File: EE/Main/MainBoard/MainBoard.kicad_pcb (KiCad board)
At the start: 2 copper layers, 141.8 x 89.6 mm, 18 parts, among them J1 Conn_02x13_Odd_Even, J2 Conn_02x13_Odd_Even, J3 Conn_02x13_Odd_Even, J4 Conn_02x13_Odd_Even, J5 Conn_02x13_Odd_Even

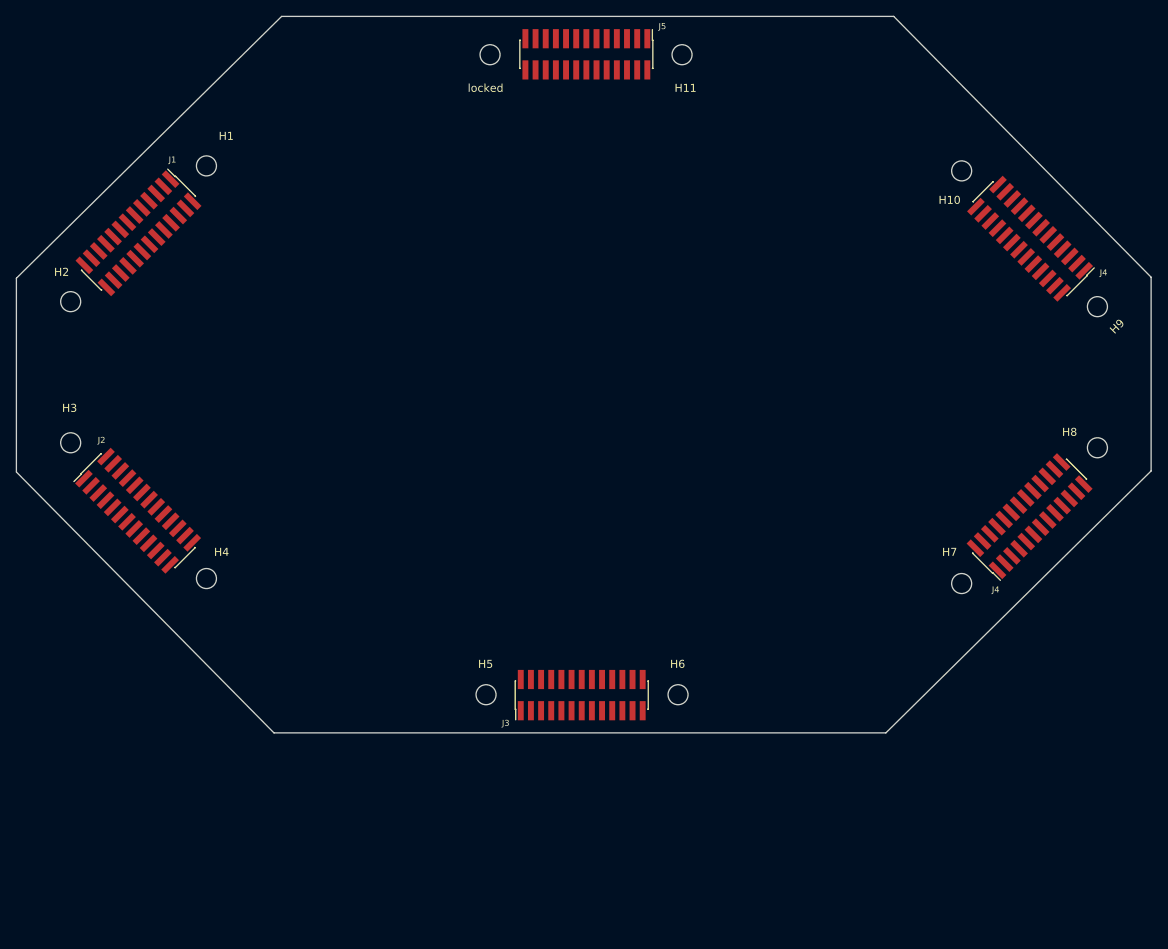
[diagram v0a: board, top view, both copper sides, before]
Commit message: Updated layout, and placement for main board
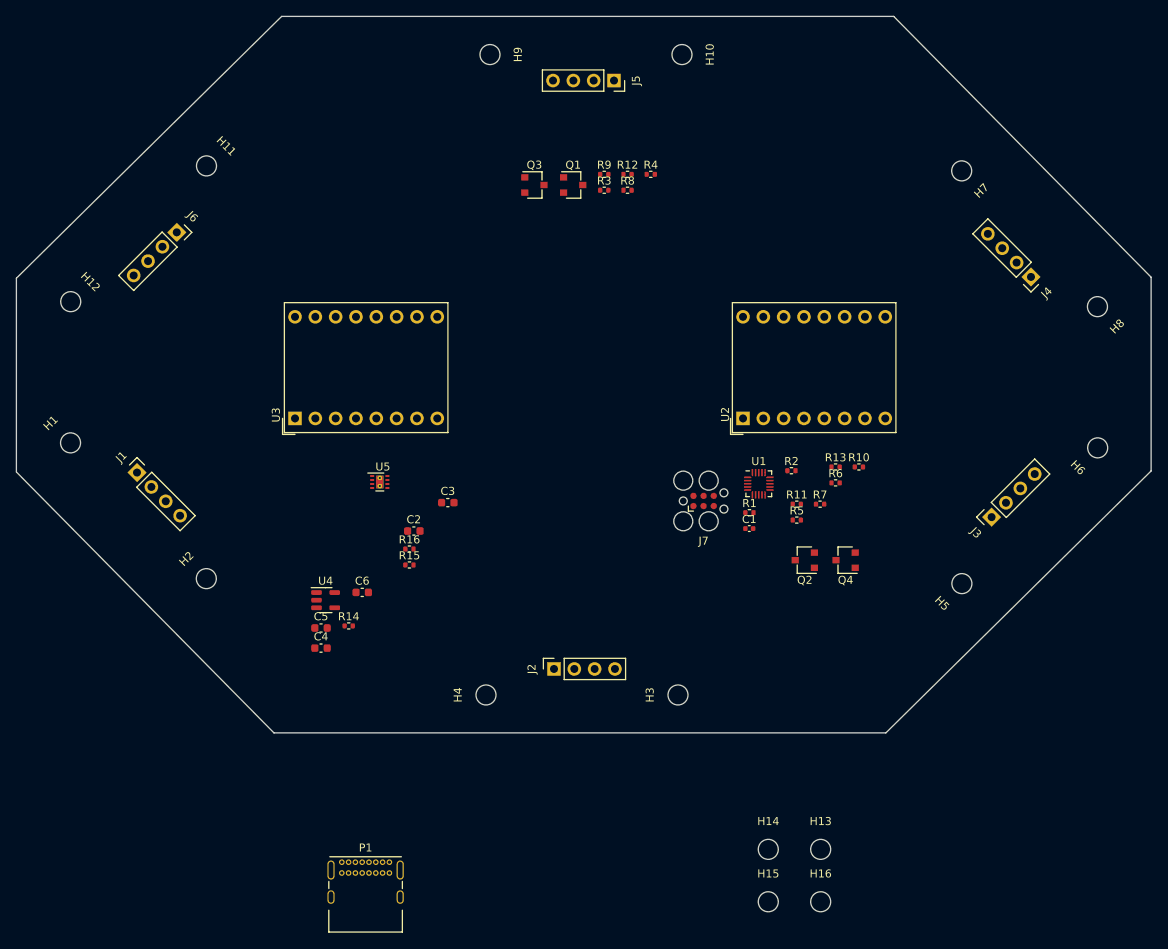
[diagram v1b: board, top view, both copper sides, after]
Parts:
- removed the J4 at (199.1, 77.8)
- removed the J4 at (199.0, 112.5)
- removed locked: MountingHole, MountingHole:MountingHole_2.5mm
- added C1: 0.1u, Capacitor_SMD:C_0402_1005Metric, F.Cu at (164.0, 114.0)
- added C2: 4.7u, Capacitor_SMD:C_0603_1608Metric, F.Cu at (122.0, 114.4)
- added C3: 4.7u, Capacitor_SMD:C_0603_1608Metric, F.Cu at (126.3, 110.8)
- added C4: 4.7u, Capacitor_SMD:C_0603_1608Metric, F.Cu at (110.4, 129.0)
- added C5: 4.7u, Capacitor_SMD:C_0603_1608Metric, F.Cu at (110.4, 126.5)
- added C6: 4.7u, Capacitor_SMD:C_0603_1608Metric, F.Cu at (115.6, 122.0)
- added H12: MountingHole, MountingHole:MountingHole_2.5mm, F.Cu at (79.1, 85.7)
- added H13: MountingHole, MountingHole:MountingHole_2.5mm, F.Cu at (172.9, 154.2)
- added H14: MountingHole, MountingHole:MountingHole_2.5mm, F.Cu at (166.3, 154.2)
- added H15: MountingHole, MountingHole:MountingHole_2.5mm, F.Cu at (166.3, 160.7)
- added H16: MountingHole, MountingHole:MountingHole_2.5mm, F.Cu at (172.9, 160.7)
- added J4: Conn_01x04_Male, Connector_PinSocket_2.54mm:PinSocket_1x04_P2.54mm_Vertical, F.Cu at (199.2, 82.6)
- added J6: Conn_01x04_Male, Connector_PinSocket_2.54mm:PinSocket_1x04_P2.54mm_Vertical, F.Cu at (92.4, 77.0)
- added J7: TAG_CONNECT, Connector:Tag-Connect_TC2030-IDC-FP_2x03_P1.27mm_Vertical, F.Cu at (158.2, 110.6)
- added P1: USB_C_Plug_USB2.0, Connector_USB:USB_C_Receptacle_GCT_USB4085, F.Cu at (113.0, 155.8)
- added Q1: 2N7002NXAKR, Package_TO_SOT_SMD:SC-59, F.Cu at (141.9, 71.1)
- added Q2: 2N7002NXAKR, Package_TO_SOT_SMD:SC-59, F.Cu at (170.9, 118.0)
- added Q3: 2N7002NXAKR, Package_TO_SOT_SMD:SC-59, F.Cu at (137.1, 71.1)
- added Q4: 2N7002NXAKR, Package_TO_SOT_SMD:SC-59, F.Cu at (176.0, 118.0)
- added R1: 4.7k, Resistor_SMD:R_0402_1005Metric, F.Cu at (164.0, 112.1)
- added R10: 560, Resistor_SMD:R_0402_1005Metric, F.Cu at (177.7, 106.3)
- added R11: 560, Resistor_SMD:R_0402_1005Metric, F.Cu at (169.9, 111.0)
- added R12: 560, Resistor_SMD:R_0402_1005Metric, F.Cu at (148.7, 69.8)
- added R13: 560, Resistor_SMD:R_0402_1005Metric, F.Cu at (174.8, 106.3)
- added R14: 20k, Resistor_SMD:R_0402_1005Metric, F.Cu at (113.9, 126.2)
- added R15: 2k, Resistor_SMD:R_0402_1005Metric, F.Cu at (121.5, 118.6)
- added R16: 100k, Resistor_SMD:R_0402_1005Metric, F.Cu at (121.5, 116.6)
- added R2: 4.7k, Resistor_SMD:R_0402_1005Metric, F.Cu at (169.2, 106.8)
- added R3: 10k, Resistor_SMD:R_0402_1005Metric, F.Cu at (145.8, 71.8)
- added R4: 10k, Resistor_SMD:R_0402_1005Metric, F.Cu at (151.7, 69.8)
- added R5: 10k, Resistor_SMD:R_0402_1005Metric, F.Cu at (169.9, 113.0)
- added R6: 10k, Resistor_SMD:R_0402_1005Metric, F.Cu at (174.8, 108.3)
- added R7: 560, Resistor_SMD:R_0402_1005Metric, F.Cu at (172.8, 111.0)
- added R8: 560, Resistor_SMD:R_0402_1005Metric, F.Cu at (148.7, 71.8)
- added R9: 560, Resistor_SMD:R_0402_1005Metric, F.Cu at (145.8, 69.8)
- added U1: STM32C011F4U6TR, Package_DFN_QFN:UQFN-20_3x3mm_P0.4mm, F.Cu at (165.2, 108.5)
- added U2: DA04-11EWA, Display_7Segment:DA04-11SURKWA, F.Cu at (163.2, 100.3)
- added U3: DA04-11GWA, Display_7Segment:DA04-11CGKWA, F.Cu at (107.2, 100.3)
- added U4: MCP73832-2-OT, Package_TO_SOT_SMD:SOT-23-5, F.Cu at (111.0, 123.0)
- added U5: TPS62172DSG, Package_SON:WSON-8-1EP_2x2mm_P0.5mm_EP0.9x1.6mm_ThermalVias, F.Cu at (117.8, 108.2)
- J1, J2, J3, J5: value Conn_02x13_Odd_Even -> Conn_01x04_Male; footprint Connector_PinHeader_1.27mm:PinHeader_2x13_P1.27mm_Vertical_SMD -> Connector_PinSocket_2.54mm:PinSocket_1x04_P2.54mm_Vertical
- moved H9 82.2 mm to (131.5, 54.8), turned to -90 degrees
- moved H3 82.2 mm to (155.1, 134.8), turned to 90 degrees
- moved H5 61.1 mm to (190.5, 120.9), turned to 135 degrees
- moved H11 61.0 mm to (96.1, 68.7), turned to -45 degrees
- moved H6 60.9 mm to (207.5, 104.0), turned to 135 degrees
- moved J3 55.9 mm to (194.3, 112.6), turned to 135 degrees
- moved J2 55.6 mm to (139.6, 131.6), turned to 90 degrees
- moved H7 51.6 mm to (190.5, 69.3), turned to -135 degrees
- moved H1 38.6 mm to (79.1, 103.3), turned to 45 degrees
- moved H2 38.5 mm to (96.1, 120.3), turned to 45 degrees
- moved H10 37.9 mm to (155.6, 54.8), turned to -90 degrees
- moved H4 37.9 mm to (131.1, 134.8), turned to 90 degrees
- moved J1 29.9 mm to (87.4, 107.1), turned to 45 degrees
- moved H8 17.6 mm to (207.5, 86.3), turned to -135 degrees
- moved J5 4.76 mm to (147.0, 58.0)
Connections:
- J1 pad 1: (no net) -> VCC
- J1 pad 2: (no net) -> /SCL
- J1 pad 3: (no net) -> /SDA
- J1 pad 4: (no net) -> GND
- J2 pad 1: (no net) -> VCC
- J2 pad 2: (no net) -> /SCL
- J2 pad 3: (no net) -> /SDA
- J2 pad 4: (no net) -> GND
- J3 pad 1: (no net) -> VCC
- J3 pad 2: (no net) -> /SCL
- J3 pad 3: (no net) -> /SDA
- J3 pad 4: (no net) -> GND
- J5 pad 1: (no net) -> VCC
- J5 pad 2: (no net) -> /SCL
- J5 pad 3: (no net) -> /SDA
- J5 pad 4: (no net) -> GND

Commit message: Routed PCB, Need SCL/SDA still
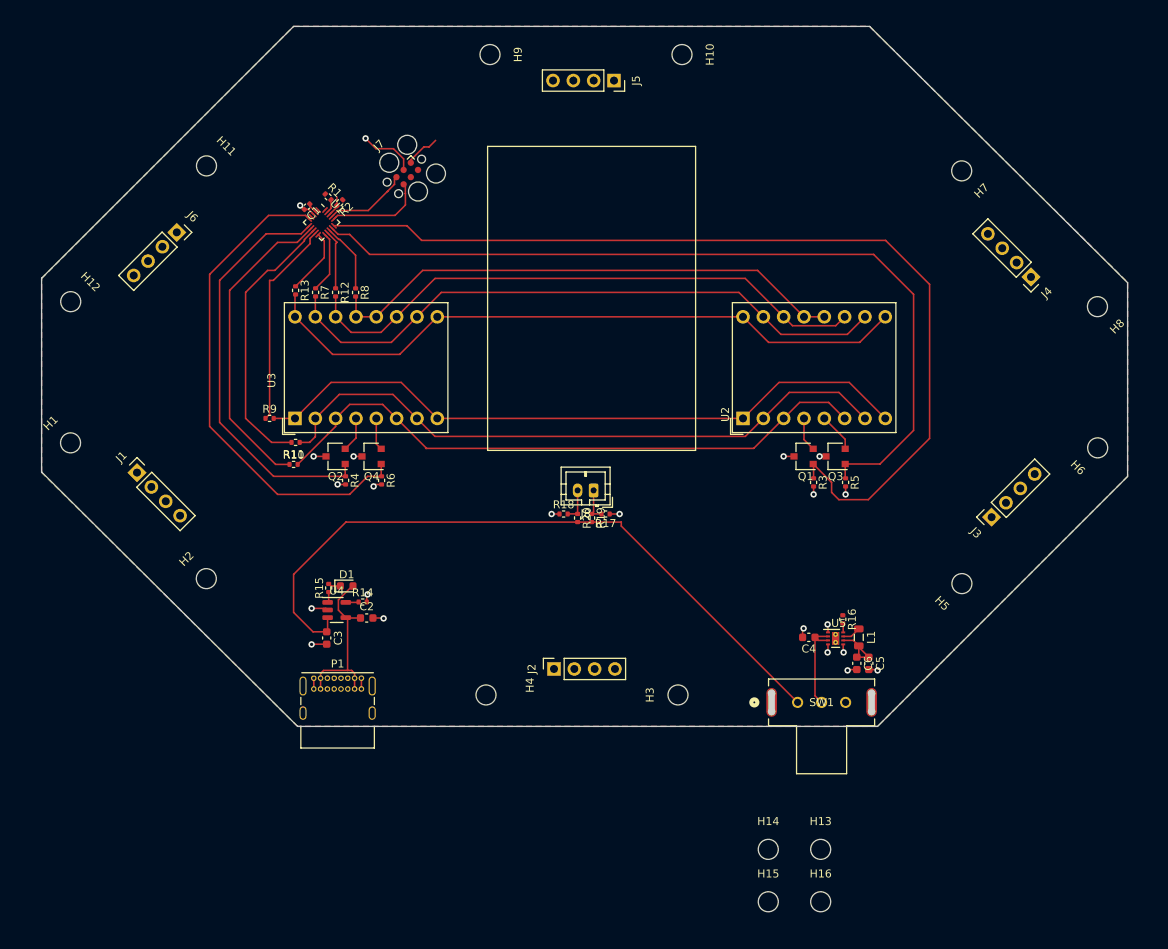
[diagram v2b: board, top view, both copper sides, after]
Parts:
- added D1: LED, LED_SMD:LED_0603_1608Metric, F.Cu at (113.6, 121.2)
- added J8: Conn_01x02_Male, Connector_JST:JST_PH_B2B-PH-K_1x02_P2.00mm_Vertical, F.Cu at (144.5, 109.3)
- added L1: 2.2u, Inductor_SMD:L_0805_2012Metric, F.Cu at (177.7, 127.7)
- added R17: 0, Resistor_SMD:R_0402_1005Metric, F.Cu at (146.0, 112.2)
- added R18: 0, Resistor_SMD:R_0402_1005Metric, F.Cu at (140.8, 112.2)
- added R19: 0, Resistor_SMD:R_0402_1005Metric, F.Cu at (144.2, 112.7)
- added R20: 0, Resistor_SMD:R_0402_1005Metric, F.Cu at (142.5, 112.7)
- added SW1: EG1206A, Library:EG1206A_EWI, F.Cu at (170.0, 135.8)
- moved R13 71.0 mm to (107.2, 84.3), turned to -90 degrees
- moved R10 70.7 mm to (107.0, 106.0)
- moved C5 68.6 mm to (178.9, 130.9), turned to -90 degrees
- moved R7 68.4 mm to (109.8, 84.5), turned to -90 degrees
- moved C1 68.4 mm to (108.7, 73.8), turned to -135 degrees
- moved R1 65.8 mm to (111.3, 72.6), turned to -45 degrees
- moved R2 65.7 mm to (112.8, 73.3), turned to -135 degrees
- moved U1 63.7 mm to (110.5, 75.8), turned to -45 degrees
- moved R11 63.1 mm to (107.2, 103.3)
- moved C6 62.5 mm to (177.4, 130.9), turned to -90 degrees
- moved C4 61.0 mm to (171.4, 127.7), turned to 180 degrees
- moved Q4 60.7 mm to (116.8, 105.0)
- moved U5 60.2 mm to (174.8, 127.8)
- moved Q2 60.1 mm to (112.2, 105.0)
- moved R6 56.8 mm to (118.0, 108.0), turned to -90 degrees
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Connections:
- U1 pad 10: /Display/F_EN -> /Display/G_EN
- U1 pad 11: /Display/G_EN -> /Display/A_EN
- U1 pad 12: /Display/D1_R_EN -> /Display/F_EN
- U1 pad 13: /Display/D2_R_EN -> /Display/B_EN
- U1 pad 14: /Display/D1_G_EN -> /Display/D2_R_EN
- U1 pad 15: /Display/D2_G_EN -> /Display/D1_R_EN
- U1 pad 5: /Display/A_EN -> /Display/D2_G_EN
- U1 pad 6: /Display/B_EN -> /Display/D1_G_EN
- U1 pad 7: /Display/C_EN -> /Display/D_EN
- U1 pad 8: /Display/D_EN -> /Display/E_EN
- U1 pad 9: /Display/E_EN -> /Display/C_EN
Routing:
- net /Display/D1_R_EN: track 0.00 -> 118.9 mm
- net /Display/D2_R_EN: track 0.00 -> 105.3 mm
- net /Power/VBAT: track 0.00 -> 87.1 mm
- net /Display/C: track 0.00 -> 83.9 mm
- net /Display/G: track 0.00 -> 83.1 mm
- net /Display/E: track 0.00 -> 80.3 mm
- net /Display/A: track 0.00 -> 78.3 mm
- net /Display/D: track 0.00 -> 77.7 mm
- net /Display/F: track 0.00 -> 72.7 mm
- net /Display/B: track 0.00 -> 65.9 mm
- net /Display/D2_G_EN: track 0.00 -> 62.2 mm
- net /Display/D1_G_EN: track 0.00 -> 51.9 mm
- net /Display/D_EN: track 0.00 -> 39.3 mm
- net GND: track 0.00 -> 36.0 mm, vias 0 -> 22
- net /Display/E_EN: track 0.00 -> 34.5 mm
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- added copper zone on B.Cu, net GND
- added copper zone on F.Cu, net VCC
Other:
- board size 141.8 x 89.6 mm -> 135.8 x 87.5 mm
